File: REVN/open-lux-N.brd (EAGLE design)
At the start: 53 x 68.6 mm, 71 parts, among them IC2 MCP73831, IC3 ATMEGA32U4-AU, IC4 MCP1700-33, J2 EG1206, Q1 BSS123, Q4 BSS123, T1 FDN340P, T2 FDN340P, X2 USBSMD, X3 8MHz

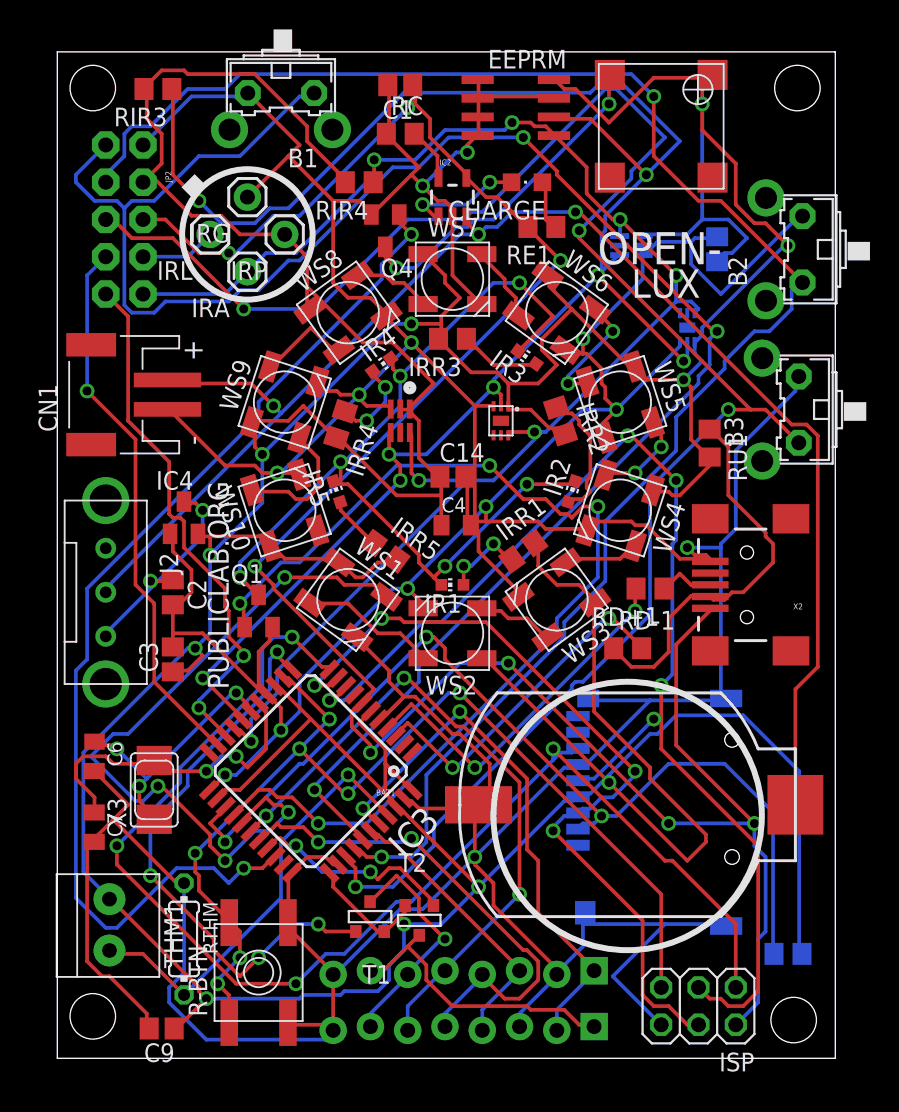
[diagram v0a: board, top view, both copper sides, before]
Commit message: update
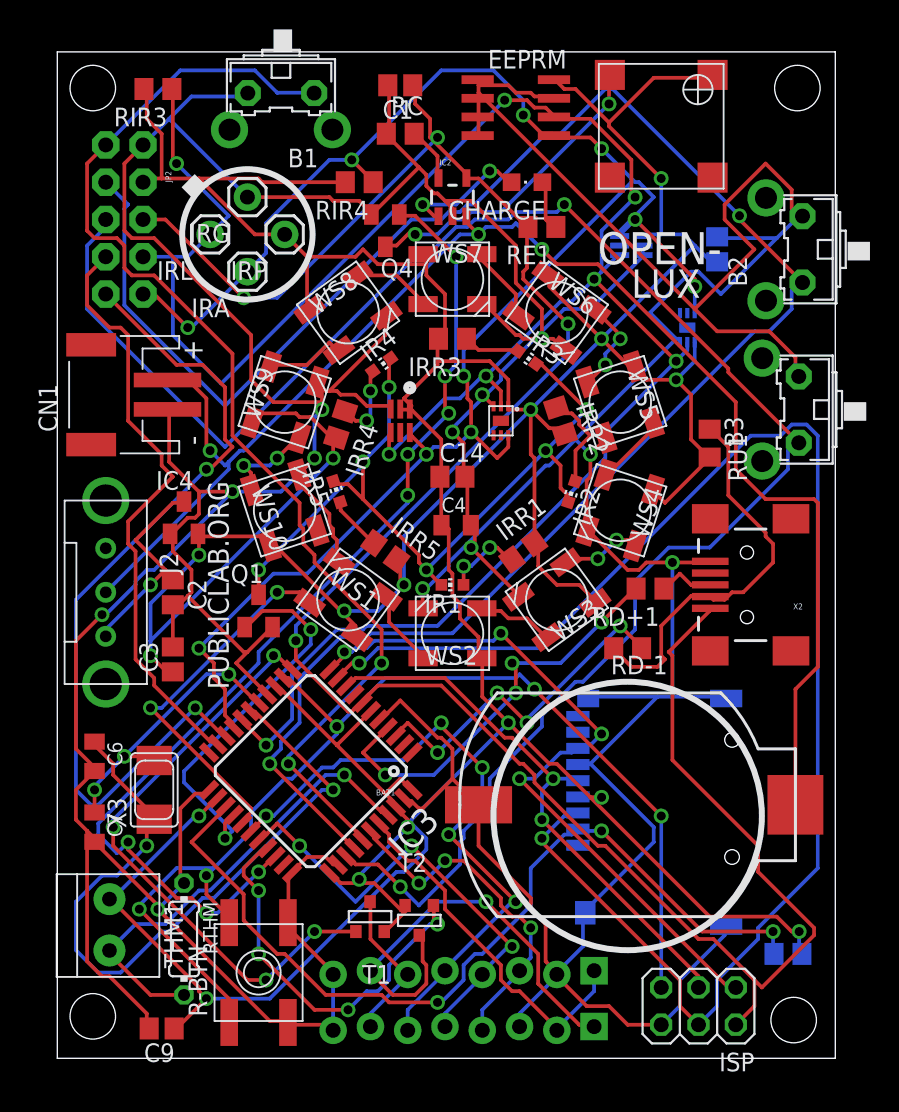
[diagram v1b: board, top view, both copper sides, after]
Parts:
- turned IR2 to 162 degrees
- turned IR3 to 234 degrees
- turned WS1 to 144 degrees
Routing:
- net VCC: track 441.8 -> 372.2 mm, vias 11 -> 16
- net A2: track 128.8 -> 79.7 mm, vias 3 -> 2
- net MOSI: track 55.8 -> 104.2 mm, vias 4 -> 2
- net SCK: track 84.3 -> 37.9 mm, vias 5 -> 2
- net D12: track 70.6 -> 26.7 mm, vias 4 -> 2
- net GND: track 464.8 -> 504.2 mm, vias 13 -> 12
- net MISO: track 88.6 -> 50.1 mm
- net N$3: track 18.3 -> 51.3 mm, vias 3 -> 2
- net D6: track 49.2 -> 25.3 mm, vias 4 -> 2
- net RXD: track 36.3 -> 57.2 mm
- net SCL: track 132.2 -> 152.4 mm
- net A1: track 115.0 -> 133.7 mm
- net SDA: track 107.8 -> 123.7 mm, vias 7 -> 10
- net A4: track 37.5 -> 24.9 mm, vias 2 -> 0
- net D10: track 14.4 -> 26.8 mm, vias 2 -> 4
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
